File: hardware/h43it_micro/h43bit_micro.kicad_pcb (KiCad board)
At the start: 2 copper layers, 39.2 x 39.2 mm, 25 parts, among them J1 Conn_01x04_Pin, SW1 SW_Push, U1 ATtiny414-SS

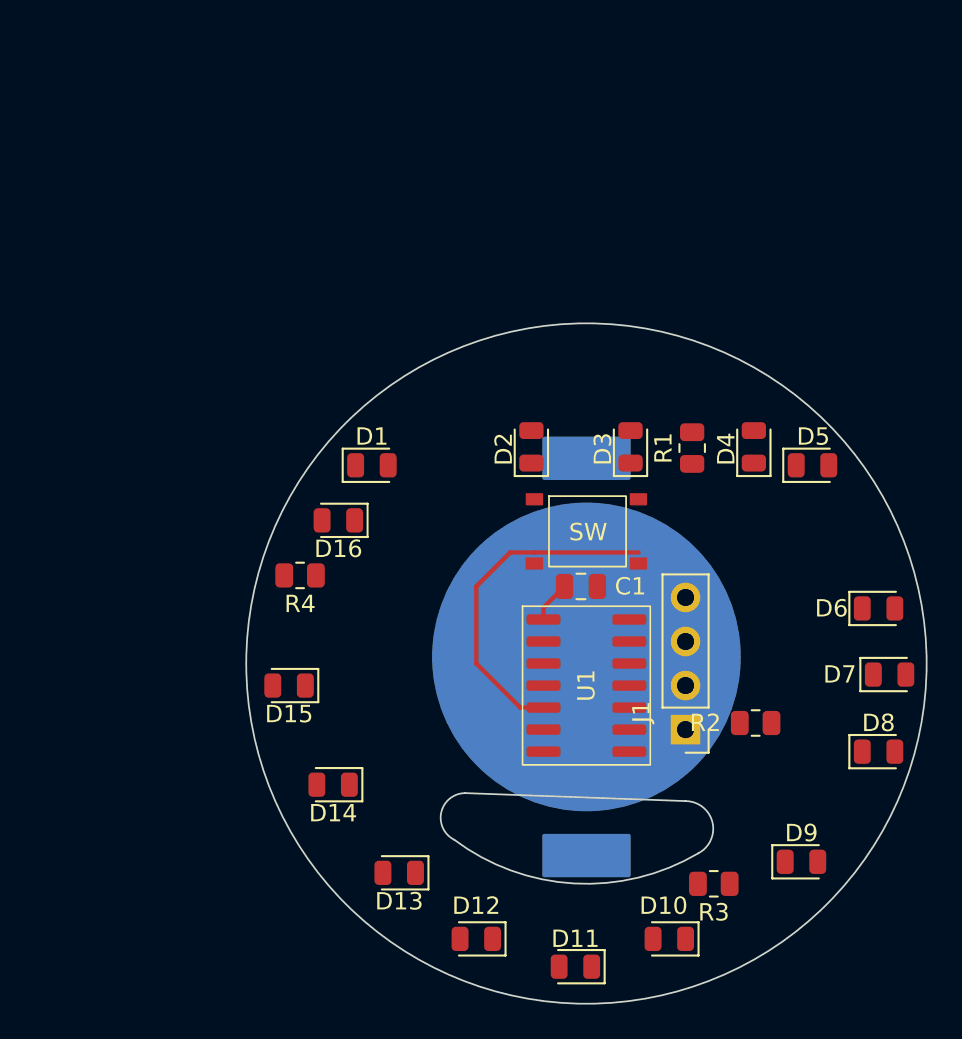
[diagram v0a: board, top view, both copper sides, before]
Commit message: circular tracks
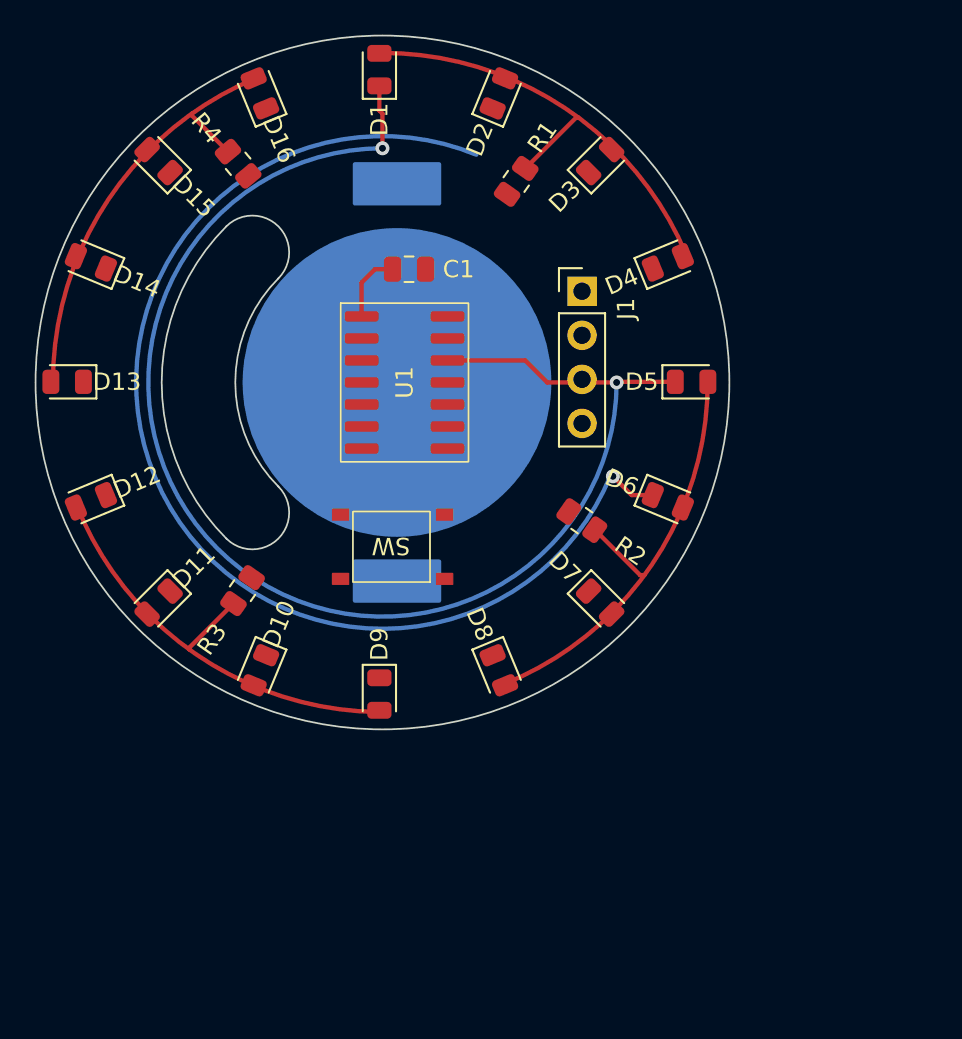
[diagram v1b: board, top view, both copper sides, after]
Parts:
- moved D13 34.2 mm to (81.8, 100.0)
- moved D12 33.6 mm to (83.2, 106.9), turned to -157.5 degrees
- moved D14 33.2 mm to (83.2, 93.1), turned to 157.5 degrees
- moved R3 32.0 mm to (91.9, 112.0), turned to -125 degrees
- moved D11 31.9 mm to (87.1, 112.7), turned to -135 degrees
- moved D15 31.2 mm to (87.1, 87.2), turned to 135 degrees
- moved D10 28.2 mm to (92.9, 116.6), turned to -112.5 degrees
- moved D9 26.2 mm to (99.8, 118.0), turned to -90 degrees
- moved J1 26.0 mm to (111.5, 94.7), turned to 0 degrees
- moved D16 25.0 mm to (92.9, 83.3), turned to 112.5 degrees
- moved R4 24.0 mm to (91.7, 87.4), turned to 130 degrees
- moved D1 22.8 mm to (99.8, 82.0), turned to 90 degrees
- moved D8 22.4 mm to (106.7, 116.6), turned to -67.5 degrees
- moved C1 20.8 mm to (101.5, 93.5)
- moved D2 20.5 mm to (106.7, 83.3), turned to 67.5 degrees
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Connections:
- BT1 pad 1: VCC -> /N-
- BT1 pad 2: GND -> /N-
- D1 pad 1: /M- -> /N-
- D5 pad 1: /M- -> /N-
- U1 pad 12: /M- -> /N-
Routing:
- net /N-: track 0.00 -> 122.5 mm, vias 0 -> 3
- net Net-(D1-A): track 0.00 -> 26.2 mm
- net Net-(D5-A): track 0.00 -> 25.9 mm
- net Net-(D10-A): track 0.00 -> 25.8 mm
- net Net-(D13-A): track 0.00 -> 25.5 mm
- net /SW: track 19.5 -> 0.00 mm
- net VCC: track 2.41 -> 4.05 mm
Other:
- board size 39.2 x 39.2 mm -> 40 x 40 mm
